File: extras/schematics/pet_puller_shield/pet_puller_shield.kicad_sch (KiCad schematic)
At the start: 19 parts, among them J1 Jack-DC, J2 Conn_01x02, J3 Conn_01x02, J4 Conn_01x02, J5 Conn_01x04, Q1 IRF540N, U1 LM317_TO-220, U2 MX1508_module

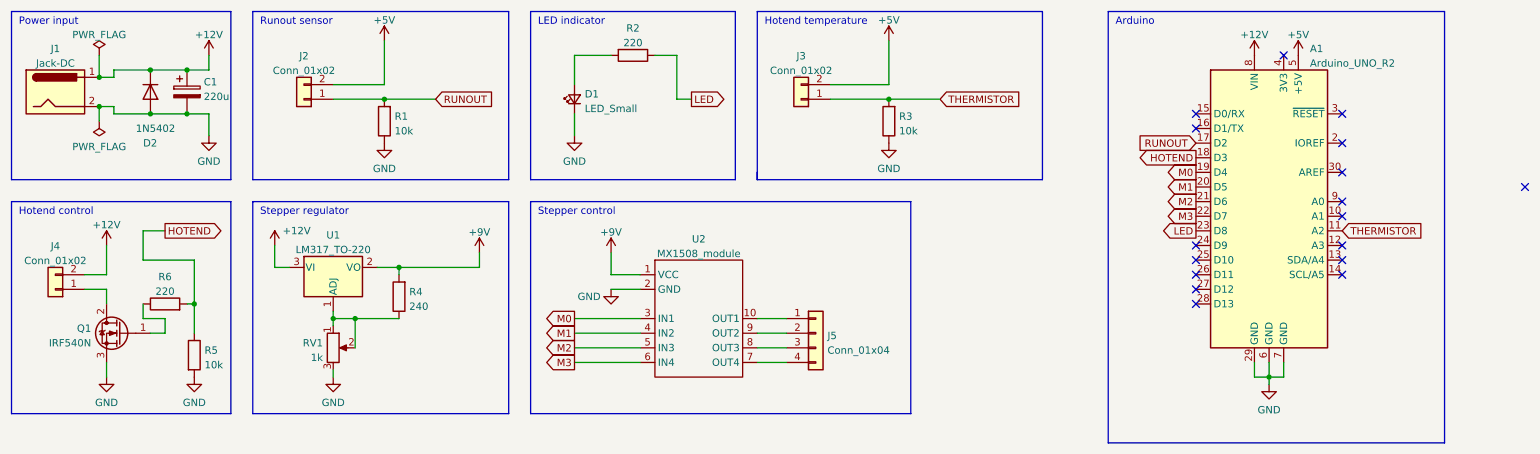
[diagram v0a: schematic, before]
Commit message: Update schematics
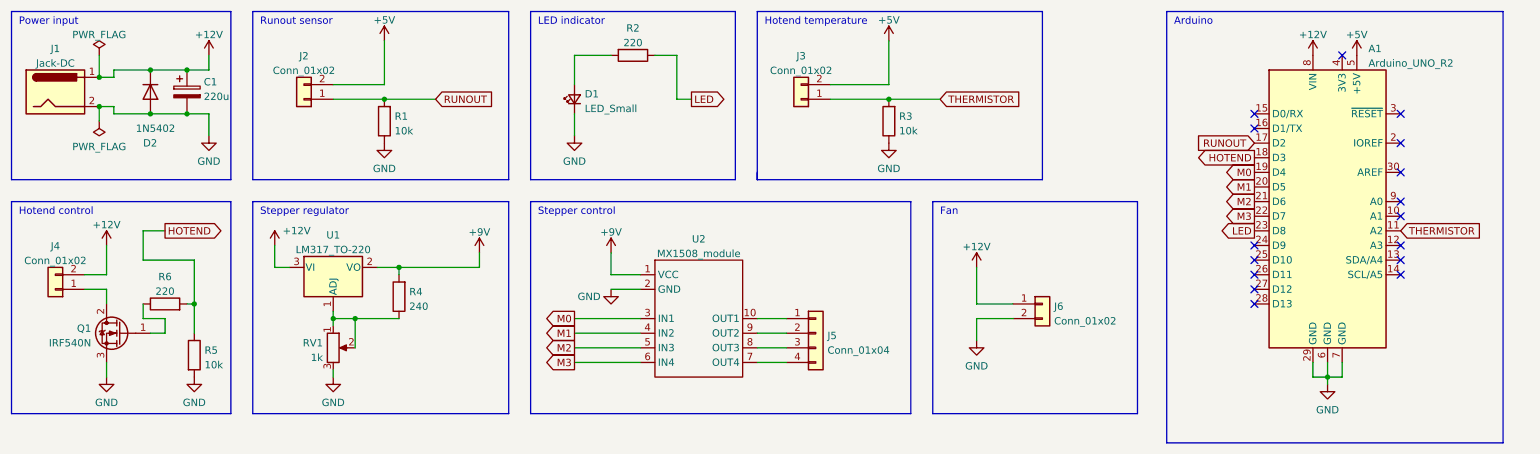
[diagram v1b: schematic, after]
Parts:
- added J6: Conn_01x02, Connector_JST:JST_EH_B2B-EH-A_1x02_P2.50mm_Vertical, symbol Connector_Generic:Conn_01x02
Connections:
- net +12V: now also J6.1 (Pin_1)
- net GND: now also J6.2 (Pin_2)
- no-connect marks 17 -> 16
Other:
- note added: "Fan"
- moved on the sheet: A1
